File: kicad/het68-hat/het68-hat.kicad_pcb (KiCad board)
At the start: 2 copper layers, 94 x 96 mm, 91 parts, among them J1 MIC1, J10 PWR, J11 PZ1, J12 PZ2, J13 PZ3, J14 PZ4, J17 UART, J2 MIC2, J3 MIC3, J4 MIC4, J5 MIC5, J6 MIC6, U1 Pico_Plus_2, U2 SN74LVC8T245, U3 SN74LVC8T245, U4 SN74LVC8T245, U5 AP2112K-1.8, U6 DRV8837C, U7 DPS310, U8 SHT40, U9 INA3221

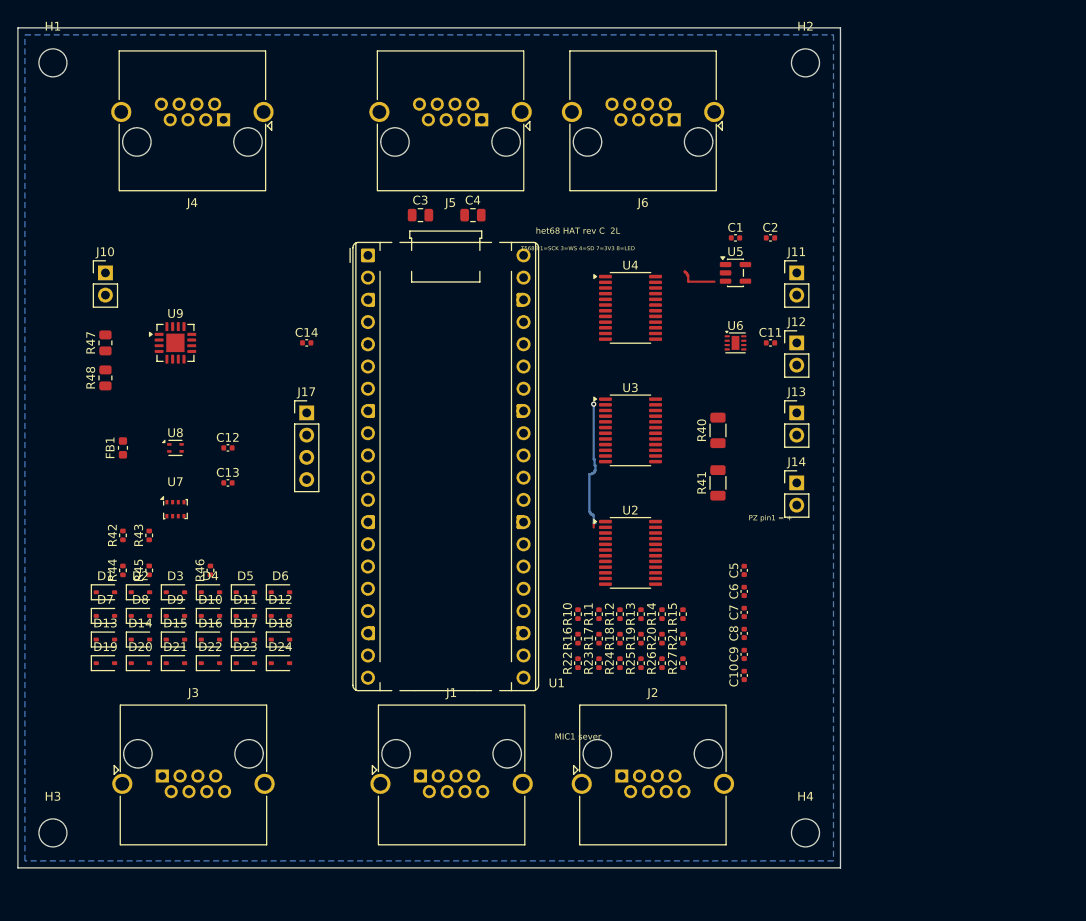
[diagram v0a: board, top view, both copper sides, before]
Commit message: Cursor: Apply local changes for cloud agent
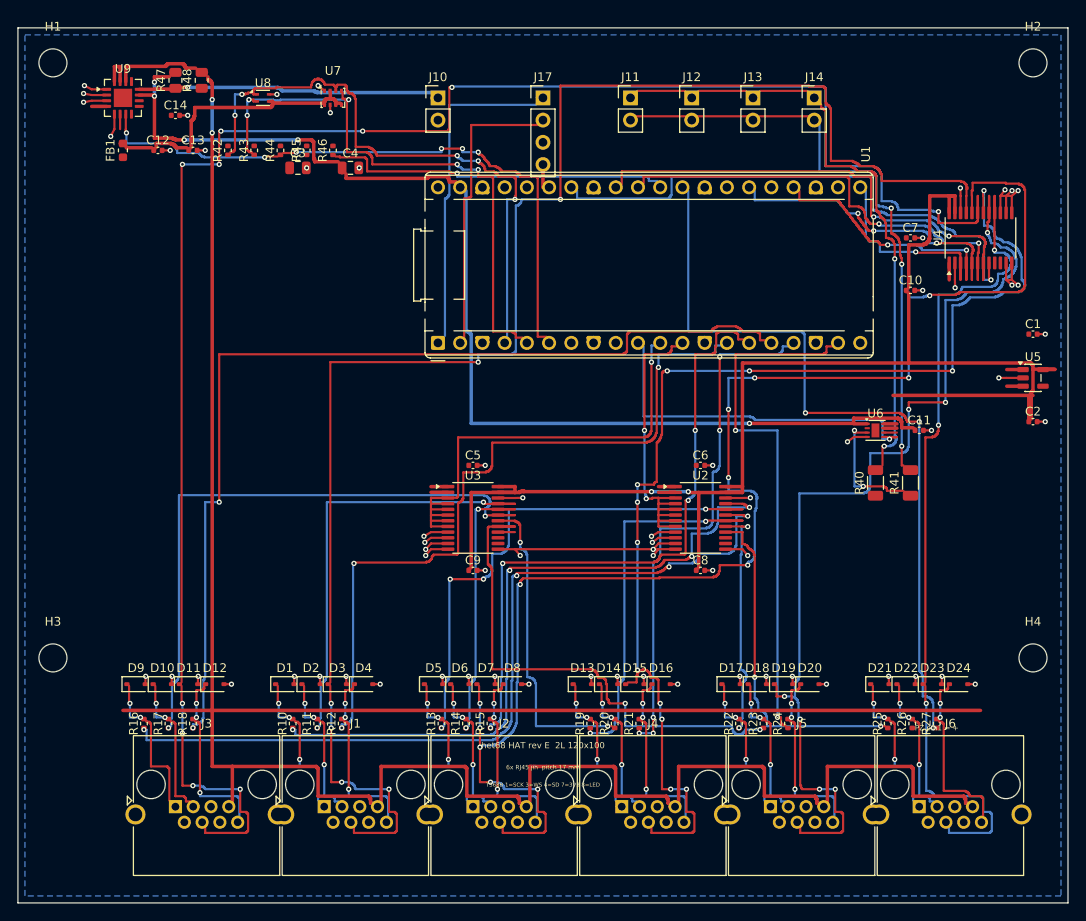
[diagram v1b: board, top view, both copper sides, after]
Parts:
- moved J4 90.7 mm to (69.0, 89.0), turned to 0 degrees
- moved J5 85.2 mm to (86.0, 89.0), turned to 0 degrees
- moved J6 83.3 mm to (103.0, 89.0), turned to 0 degrees
- moved D21 80.5 mm to (98.5, 75.0)
- moved D22 79.5 mm to (101.5, 75.0)
- moved D23 78.5 mm to (104.5, 75.0)
- moved D19 77.5 mm to (87.5, 75.0)
- moved D24 77.5 mm to (107.5, 75.0)
- moved D20 76.5 mm to (90.5, 75.0)
- moved D17 55.7 mm to (81.5, 75.0)
- moved D13 54.7 mm to (64.5, 75.0)
- moved D18 54.7 mm to (84.5, 75.0)
- moved D14 53.7 mm to (67.5, 75.0)
- moved D15 52.7 mm to (70.5, 75.0)
- moved D16 51.8 mm to (73.5, 75.0)
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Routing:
- net +3V3_MIC: track 0.00 -> 315.2 mm, vias 0 -> 2
- net SD3_18: track 0.00 -> 210.4 mm, vias 0 -> 10
- net SD1_18: track 0.00 -> 186.3 mm, vias 0 -> 6
- net SD2_18: track 0.00 -> 173.6 mm, vias 0 -> 12
- net +1V8: track 0.00 -> 163.5 mm, vias 0 -> 2
- net SD4_18: track 0.00 -> 140.8 mm, vias 0 -> 12
- net VSYS: track 0.00 -> 130.9 mm, vias 0 -> 5
- net GND: track 0.00 -> 123.4 mm, vias 0 -> 66
- net SD5_18: track 0.00 -> 118.7 mm, vias 0 -> 7
- net LED3_G: track 0.00 -> 113.6 mm, vias 0 -> 2
- net SD6_18: track 0.00 -> 99.9 mm, vias 0 -> 3
- net SCK3_B: track 0.00 -> 98.6 mm, vias 0 -> 4
- net LED6_G: track 0.00 -> 90.3 mm, vias 0 -> 3
- net LED1_G: track 0.00 -> 87.7 mm, vias 0 -> 3
- net SCK1_B: track 0.00 -> 82.1 mm, vias 0 -> 4
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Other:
- board size 94 x 96 mm -> 120 x 100 mm
- board text added: "6x RJ45 jih pitch 17 mm"
- board text added: "het68 HAT rev E 2L 120x100"
- board text removed: "MIC1 sever"
- board text removed: "het68 HAT rev C 2L"
